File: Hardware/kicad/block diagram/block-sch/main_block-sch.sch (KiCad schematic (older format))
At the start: 14 parts

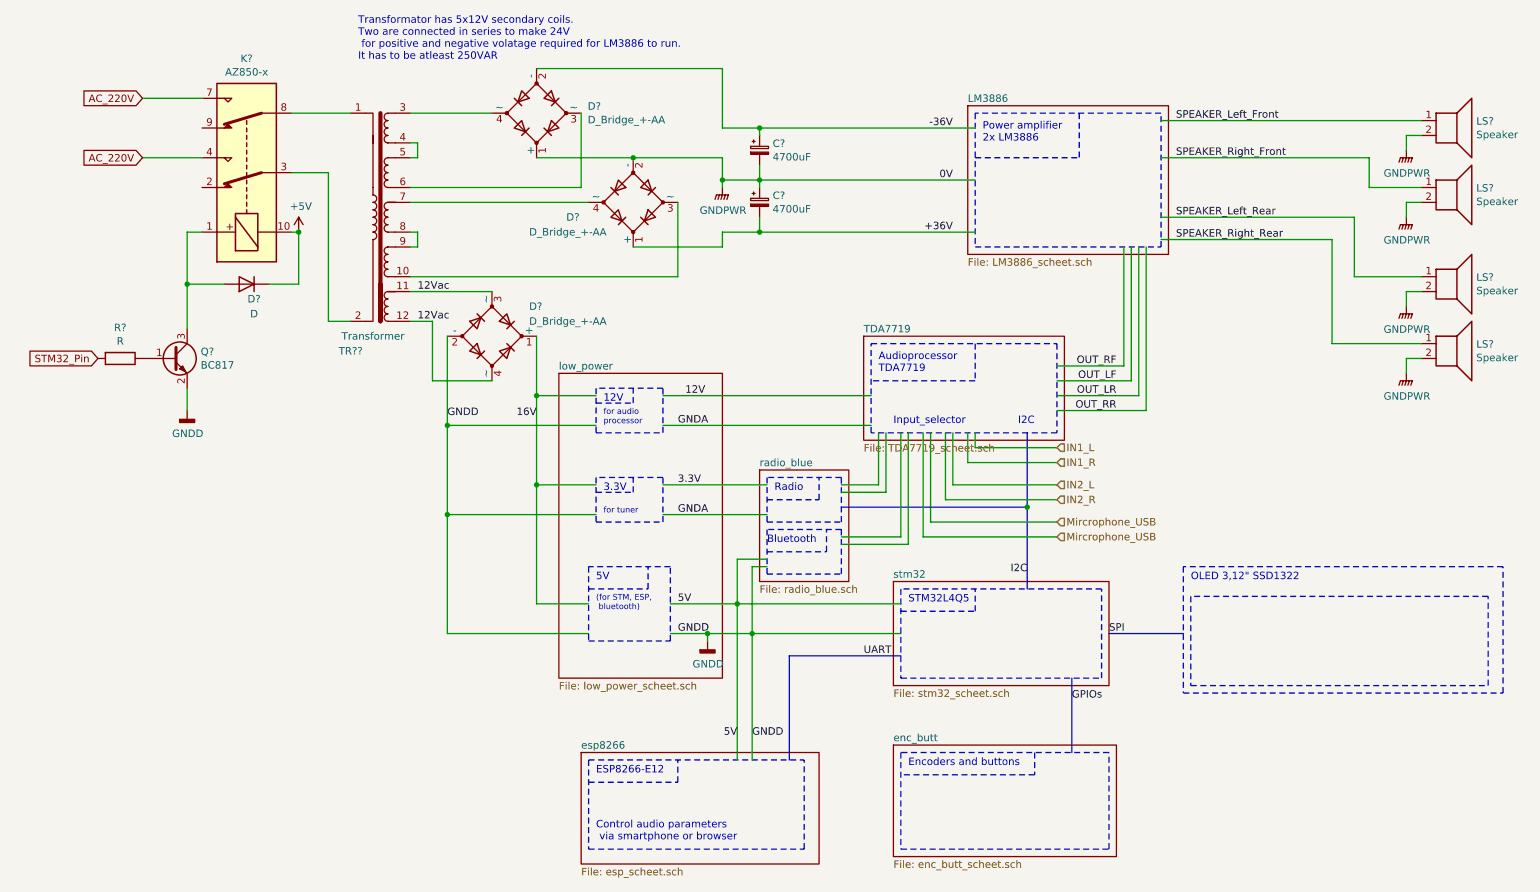
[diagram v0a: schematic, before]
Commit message: new
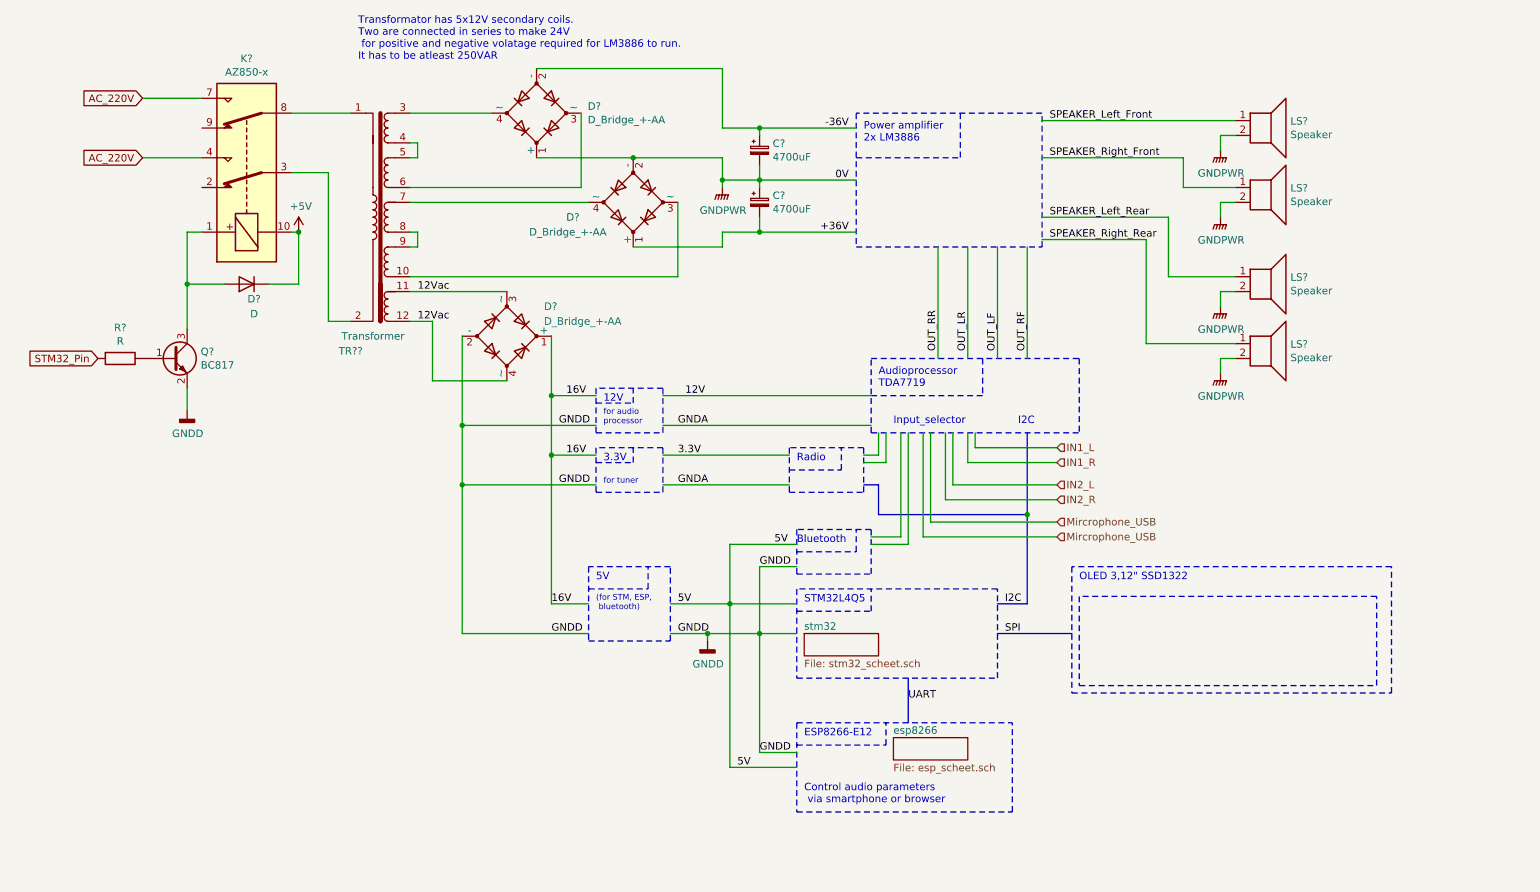
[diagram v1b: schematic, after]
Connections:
- net labels removed: GPIOs
- wire segments 122 -> 120
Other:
- note removed: "Encoders and buttons"
- moved on the sheet: D?, LS?
